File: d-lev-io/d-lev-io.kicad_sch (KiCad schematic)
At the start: 11 parts, among them J1 PJ-059A, J3 USB_C_Receptacle_USB2.0, J4 AudioJack3, J5 DIN-41524, U1 ATmega32U4-M, U4 AMS1117-5.0, U5 TPS54336ADDA

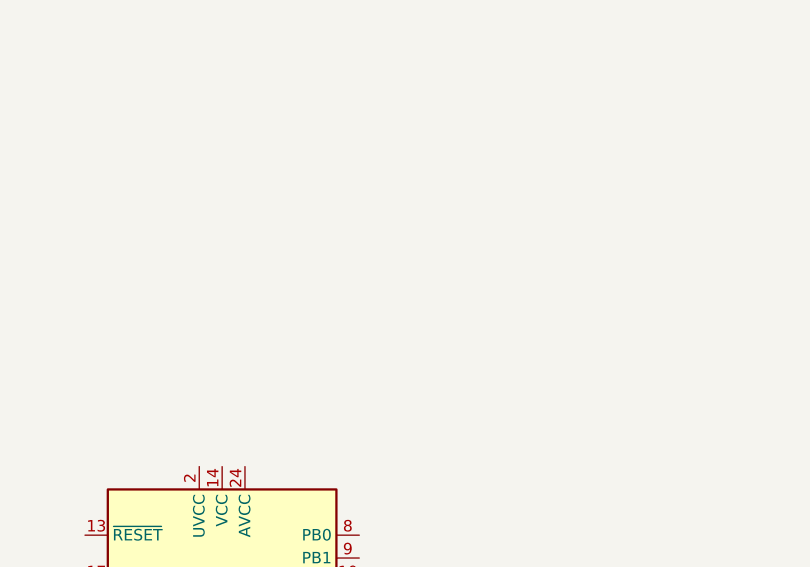
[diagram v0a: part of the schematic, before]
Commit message: Reorganized, and updates
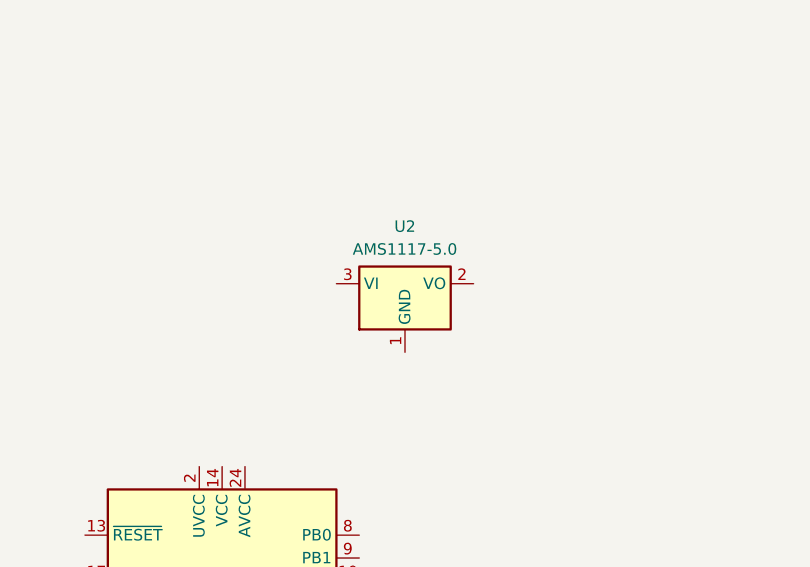
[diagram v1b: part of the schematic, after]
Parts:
- added U2: AMS1117-5.0, Package_TO_SOT_SMD:SOT-223-3_TabPin2, symbol Regulator_Linear:AMS1117-5.0
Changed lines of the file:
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@@
+    )
+  )
+  (symbol (lib_name "AMS1117-5.0_1") (lib_id "Regulator_Linear:AMS1117-5.0") (at 144.78 60.96 0) (unit 1)
+    (in_bom yes) (on_board yes) (dnp no) (fields_autoplaced)
+    (property "Reference" "U2" (at 144.78 54.61 0)
+      (effects (font (size 1.27 1.27)))
+    )
+    (property "Value" "AMS1117-5.0" (at 144.78 57.15 0)
+      (effects (font (size 1.27 1.27)))
+    )
+    (property "Footprint" "Package_TO_SOT_SMD:SOT-223-3_TabPin2" (at 144.78 55.88 0)
+      (effects (font (size 1.27 1.27)) hide)
+    )
+    (property "Datasheet" "http://www.advanced-monolithic.com/pdf/ds1117.pdf" (at 147.32 67.31 0)
+      (effects (font (size 1.27 1.27)) hide)
+    )
+    (pin "1")
+    (pin "2")
+    (pin "3")
+    (instances
+      (project "d-lev-io"
+        (path "/9261a07b-ae4a-4d72-8042-ea097cd0e5ed"
+          (reference "U2") (unit 1)
+        )
+      )
     )
   )
